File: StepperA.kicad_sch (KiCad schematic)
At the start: 19 parts

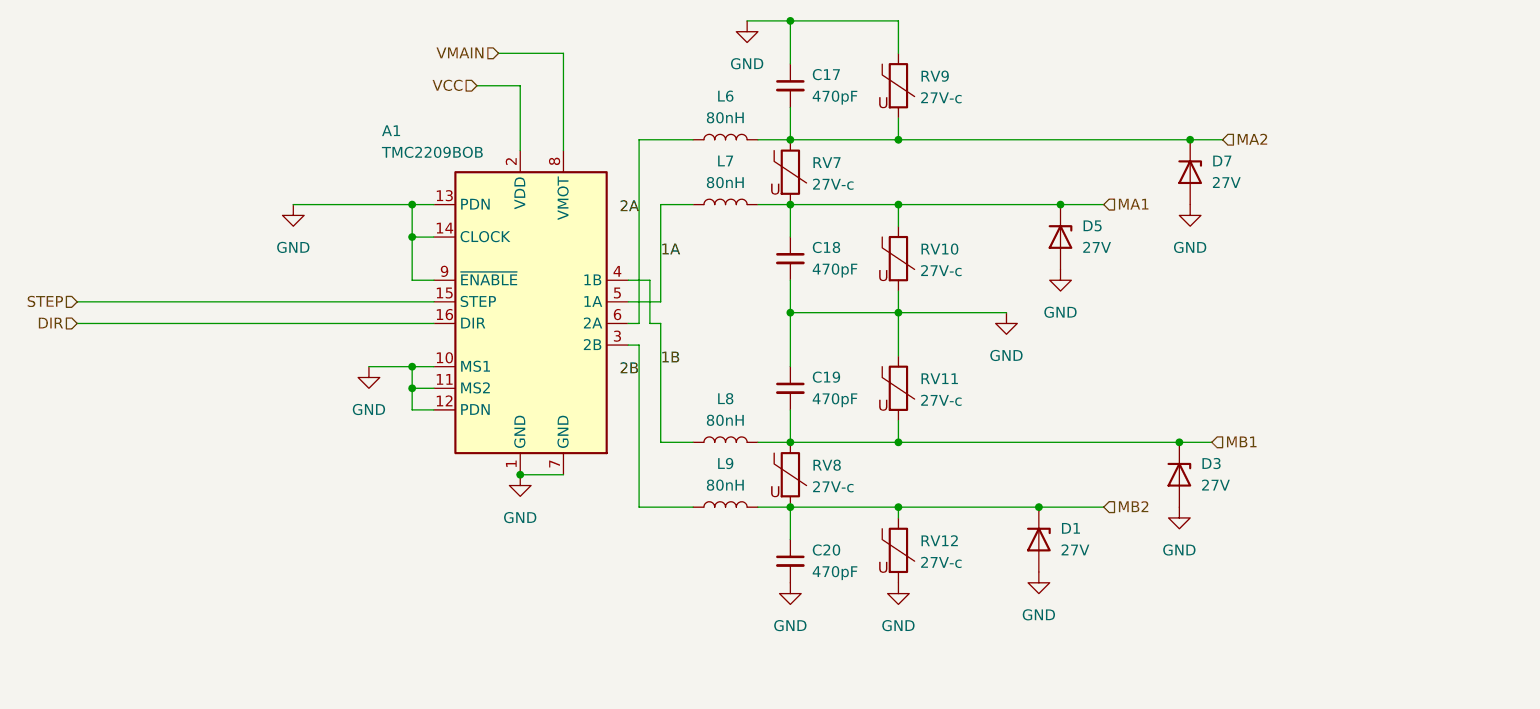
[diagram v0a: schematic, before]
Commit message: update
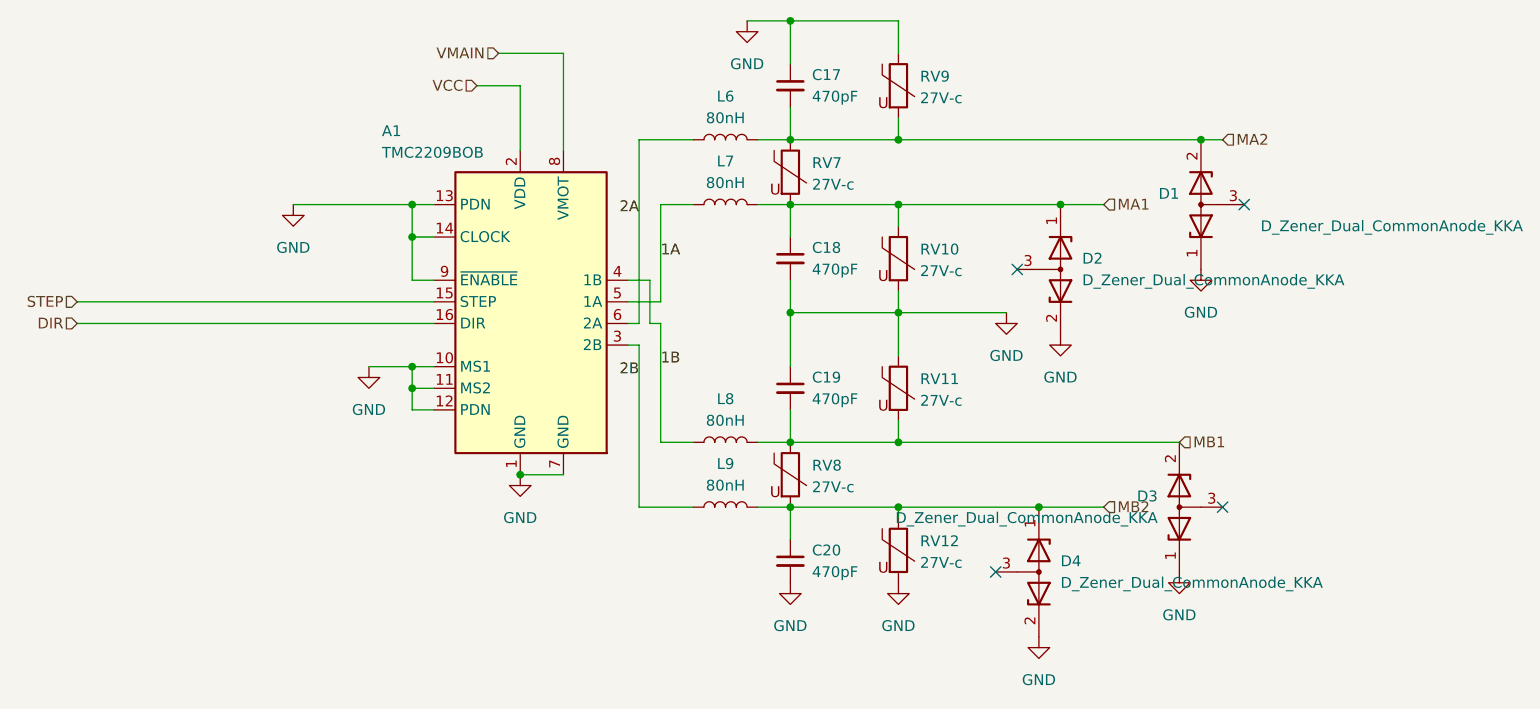
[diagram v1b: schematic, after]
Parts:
- removed D1, D3, D5, D7: 27V, Diode_SMD:D_0603_1608Metric, symbol Device:D_Zener
- added D1, D2, D3, D4: D_Zener_Dual_CommonAnode_KKA, Package_TO_SOT_SMD:TSOT-23, symbol Device:D_Zener_Dual_CommonAnode_KKA
- L6, L7, L8, L9: footprint iclr:IND_FDSD0630-H-1R0M=P3 -> Inductor_SMD:L_0603_1608Metric
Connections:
- net GND: now also D1.1 (K), D2.2 (K), D3.1 (K), D4.2 (K)
- net MA1: now also D2.1 (K)
- net MA2: now also D1.2 (K)
- net MB1: now also D3.2 (K)
- net MB2: now also D4.1 (K)
- no-connect marks 0 -> 4
